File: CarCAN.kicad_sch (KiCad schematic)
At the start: 17 parts, among them J2 CAN_OUT, U4 ADM3055E, U5 CDSOT23-T24CAN

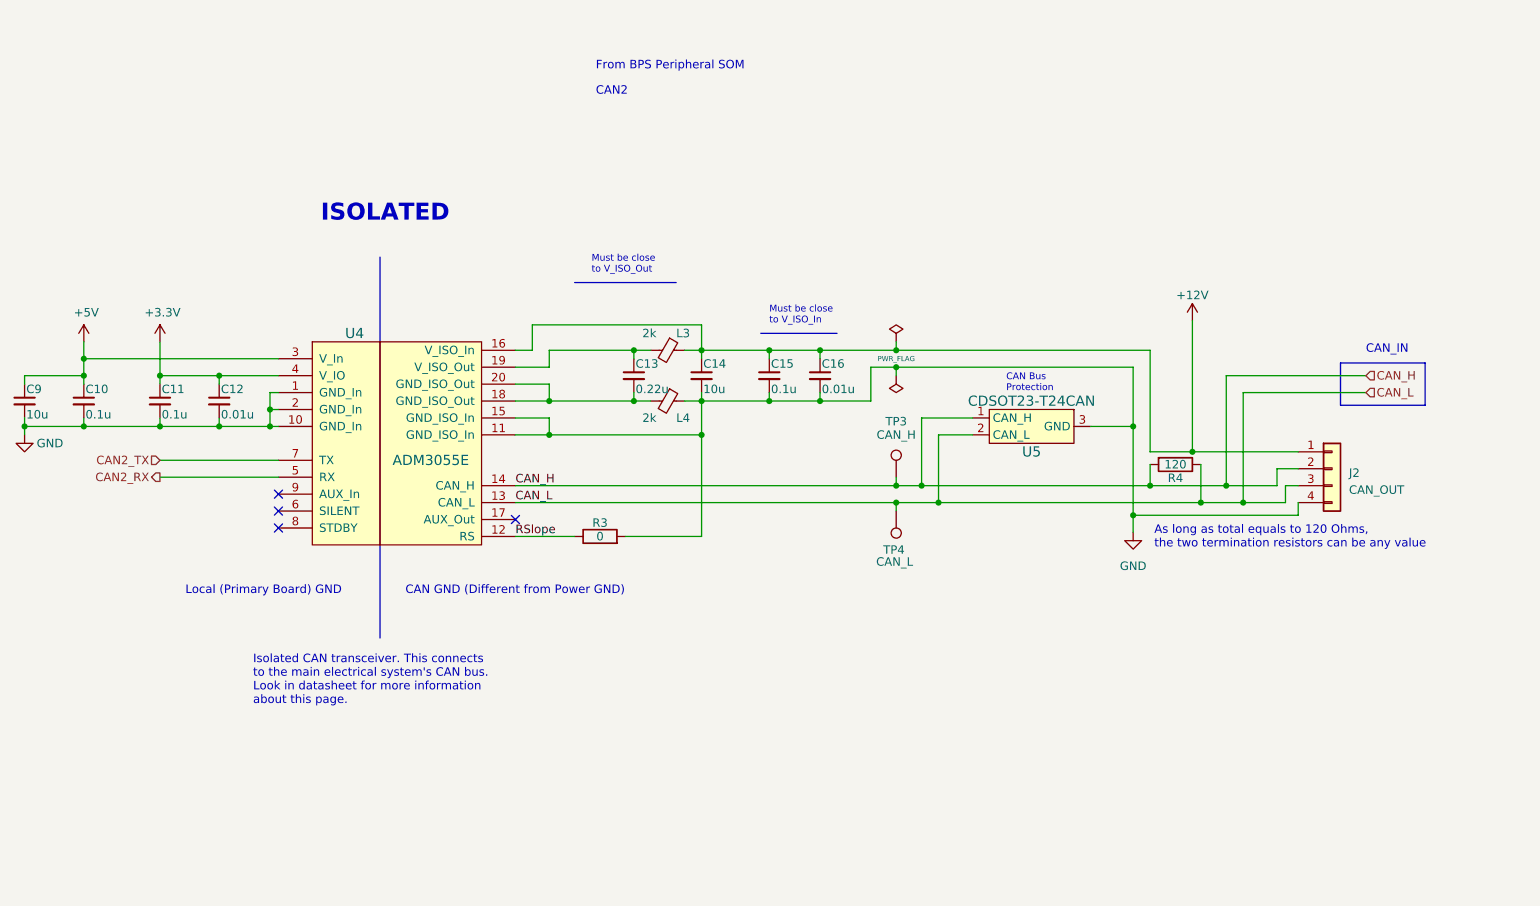
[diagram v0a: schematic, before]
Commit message: Updated pinouts and added protection circuitry for signals
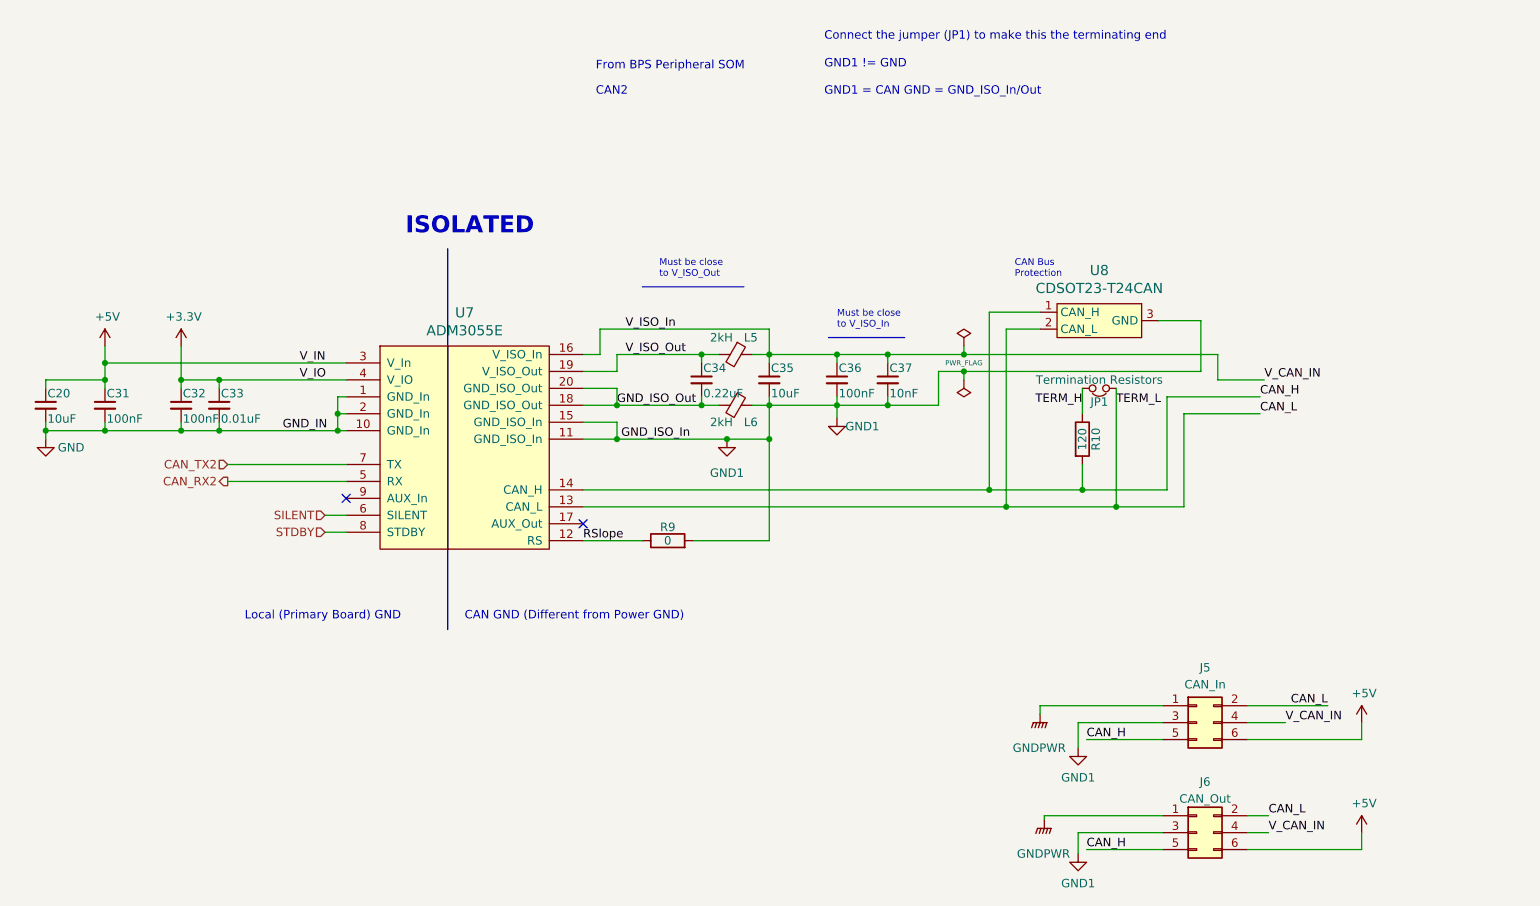
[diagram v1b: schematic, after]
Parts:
- removed C10, C11, C15: 0.1u, Capacitor_SMD:C_0805_2012Metric, symbol Device:C_Small
- removed C12, C16: 0.01u, Capacitor_SMD:C_0805_2012Metric, symbol Device:C_Small
- removed C13: 0.22u, Capacitor_SMD:C_0805_2012Metric, symbol Device:C_Small
- removed C14, C9: 10u, Capacitor_SMD:C_0805_2012Metric, symbol Device:C_Small
- removed J2: CAN_OUT, UTSVT_Connectors:Molex_MicroFit3.0_1x4xP3.00mm_PolarizingPeg_Vertical, symbol Connector_Generic:Conn_01x04
- removed L3, L4: 2k, Inductor_SMD:L_0805_2012Metric, symbol Device:FerriteBead_Small
- removed R3: 0, Resistor_SMD:R_0805_2012Metric, symbol Device:R
- removed R4: 120, Resistor_SMD:R_0805_2012Metric, symbol Device:R
- removed TP3: CAN_H, TestPoint:TestPoint_Keystone_5005-5009_Compact, symbol Connector:TestPoint
- removed TP4: CAN_L, TestPoint:TestPoint_Keystone_5005-5009_Compact, symbol Connector:TestPoint
- removed U4: ADM3055E, UTSVT_ICs:SOIC-20W_7.5x15.4mm_Pitch1.27mm, symbol utsvt-chips:ADM3055E
- removed U5: CDSOT23-T24CAN, Package_TO_SOT_SMD:SOT-23W, symbol utsvt-chips:CDSOT23-T24CAN
- added C20, C35: 10uF, Capacitor_SMD:C_0805_2012Metric, symbol Device:C_Small
- added C31, C32, C36: 100nF, Capacitor_SMD:C_0805_2012Metric, symbol Device:C_Small
- added C33: 0.01uF, Capacitor_SMD:C_0805_2012Metric, symbol Device:C_Small
- added C34: 0.22uF, Capacitor_SMD:C_0805_2012Metric, symbol Device:C_Small
- added C37: 10nF, Capacitor_SMD:C_0805_2012Metric, symbol Device:C_Small
- added J5: CAN_In, Connector_Molex:Molex_Micro-Fit_3.0_43045-0612_2x03_P3.00mm_Vertical, symbol Connector_Generic:Conn_02x03_Odd_Even
- added J6: CAN_Out, Connector_Molex:Molex_Micro-Fit_3.0_43045-0612_2x03_P3.00mm_Vertical, symbol Connector_Generic:Conn_02x03_Odd_Even
- added JP1: Termination Resistors, Connector_PinHeader_2.54mm:PinHeader_1x02_P2.54mm_Vertical, symbol Device:Jumper_NC_Small
- added L5, L6: 2kH, Inductor_SMD:L_0805_2012Metric, symbol Device:Ferrite_Bead_Small
- added R10: 120, Resistor_SMD:R_0805_2012Metric, symbol Device:R
- added R9: 0, Resistor_SMD:R_0805_2012Metric, symbol Device:R
- added U7: ADM3055E, UTSVT_ICs:SOIC-20W_7.5x15.4mm_Pitch1.27mm, symbol Dashboard-rescue:ADM3055E-utsvt-chips
- added U8: CDSOT23-T24CAN, Package_TO_SOT_SMD:SOT-23W, symbol Dashboard-rescue:CDSOT23-T24CAN-utsvt-chips
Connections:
- net +3.3V: now also C32.1, C33.1, U7.4 (V_IO)
- net +5V: now also C20.1, C31.1, J5.6 (Pin_6), J6.6 (Pin_6), U7.3 (V_In)
- net CAN_H: now also J5.5 (Pin_5), J6.5 (Pin_5), R10.2, U7.14 (CAN_H), U8.1 (CAN_H)
- net CAN_L: now also J5.2 (Pin_2), J6.2 (Pin_2), JP1.1, U7.13 (CAN_L), U8.2 (CAN_L)
- net GND: now also C20.2, C31.2, C32.2, C33.2, U7.1 (GND_In), U7.10 (GND_In), U7.2 (GND_In)
- net RSlope: now also R9.1, U7.12 (RS)
- new net CAN_RX2: U7.5 (RX)
- new net CAN_TX2: U7.7 (TX)
- new net GND1: C35.2, C36.2, C37.2, J5.3 (Pin_3), J6.3 (Pin_3), L6.1, R9.2, U7.11 (GND_ISO_In), U7.15 (GND_ISO_In), U8.3 (GND)
- new net GNDPWR: J5.1 (Pin_1), J6.1 (Pin_1)
- new net GND_ISO_Out: C34.2, L6.2, U7.18 (GND_ISO_Out), U7.20 (GND_ISO_Out)
- new net SILENT: U7.6 (SILENT)
- new net STDBY: U7.8 (STDBY)
- new net TERM_H: JP1.2, R10.1
- new net V_CAN_IN: C35.1, C36.1, C37.1, J5.4 (Pin_4), J6.4 (Pin_4), L5.1, U7.16 (V_ISO_In)
- new net V_ISO_Out: C34.1, L5.2, U7.19 (V_ISO_Out)
- no-connect marks 4 -> 2
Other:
- note added: "Connect the jumper (JP1) to make this the terminating end"
- note added: "GND1 != GND GND1 = CAN GND = GND_ISO_In/Out"
- note removed: "As long as total equals to 120 Ohms, the two termination resistors can be any value"
- note removed: "CAN_IN"
- note removed: "Isolated CAN transceiver. This connects to the main electrical system's CAN bus. Look in datasheet for more information about this page."

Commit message: Updated power distribution design
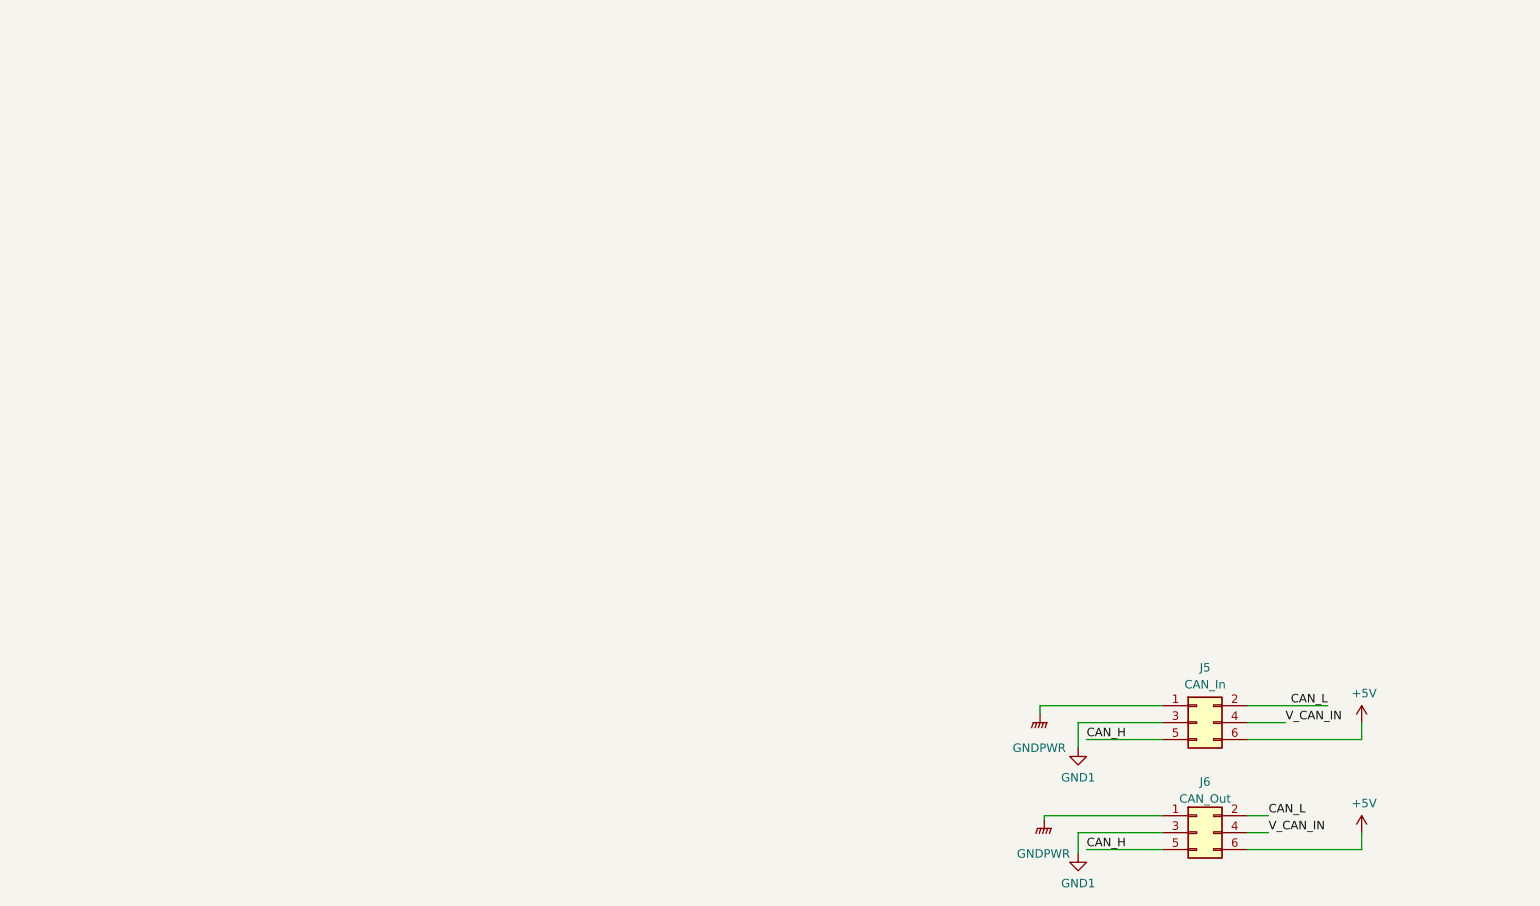
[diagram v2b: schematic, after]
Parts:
- removed C20, C35: 10uF, Capacitor_SMD:C_0805_2012Metric, symbol Device:C_Small
- removed C31, C32, C36: 100nF, Capacitor_SMD:C_0805_2012Metric, symbol Device:C_Small
- removed C33: 0.01uF, Capacitor_SMD:C_0805_2012Metric, symbol Device:C_Small
- removed C34: 0.22uF, Capacitor_SMD:C_0805_2012Metric, symbol Device:C_Small
- removed C37: 10nF, Capacitor_SMD:C_0805_2012Metric, symbol Device:C_Small
- removed JP1: Termination Resistors, Connector_PinHeader_2.54mm:PinHeader_1x02_P2.54mm_Vertical, symbol Device:Jumper_NC_Small
- removed L5, L6: 2kH, Inductor_SMD:L_0805_2012Metric, symbol Device:Ferrite_Bead_Small
- removed R10: 120, Resistor_SMD:R_0805_2012Metric, symbol Device:R
- removed R9: 0, Resistor_SMD:R_0805_2012Metric, symbol Device:R
- removed U7: ADM3055E, UTSVT_ICs:SOIC-20W_7.5x15.4mm_Pitch1.27mm, symbol Dashboard-rescue:ADM3055E-utsvt-chips
- removed U8: CDSOT23-T24CAN, Package_TO_SOT_SMD:SOT-23W, symbol Dashboard-rescue:CDSOT23-T24CAN-utsvt-chips
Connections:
- no-connect marks 2 -> 0
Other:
- note removed: "CAN Bus Protection"
- note removed: "CAN GND (Different from Power GND)"
- note removed: "CAN2"
- note removed: "Connect the jumper (JP1) to make this the terminating end"
- note removed: "From BPS Peripheral SOM"
- note removed: "GND1 != GND GND1 = CAN GND = GND_ISO_In/Out"
- note removed: "ISOLATED"
- note removed: "Local (Primary Board) GND"
- note removed: "Must be close to V_ISO_In"
- note removed: "Must be close to V_ISO_Out"

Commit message: Updated CAN circuitry and used new power protection PMOS
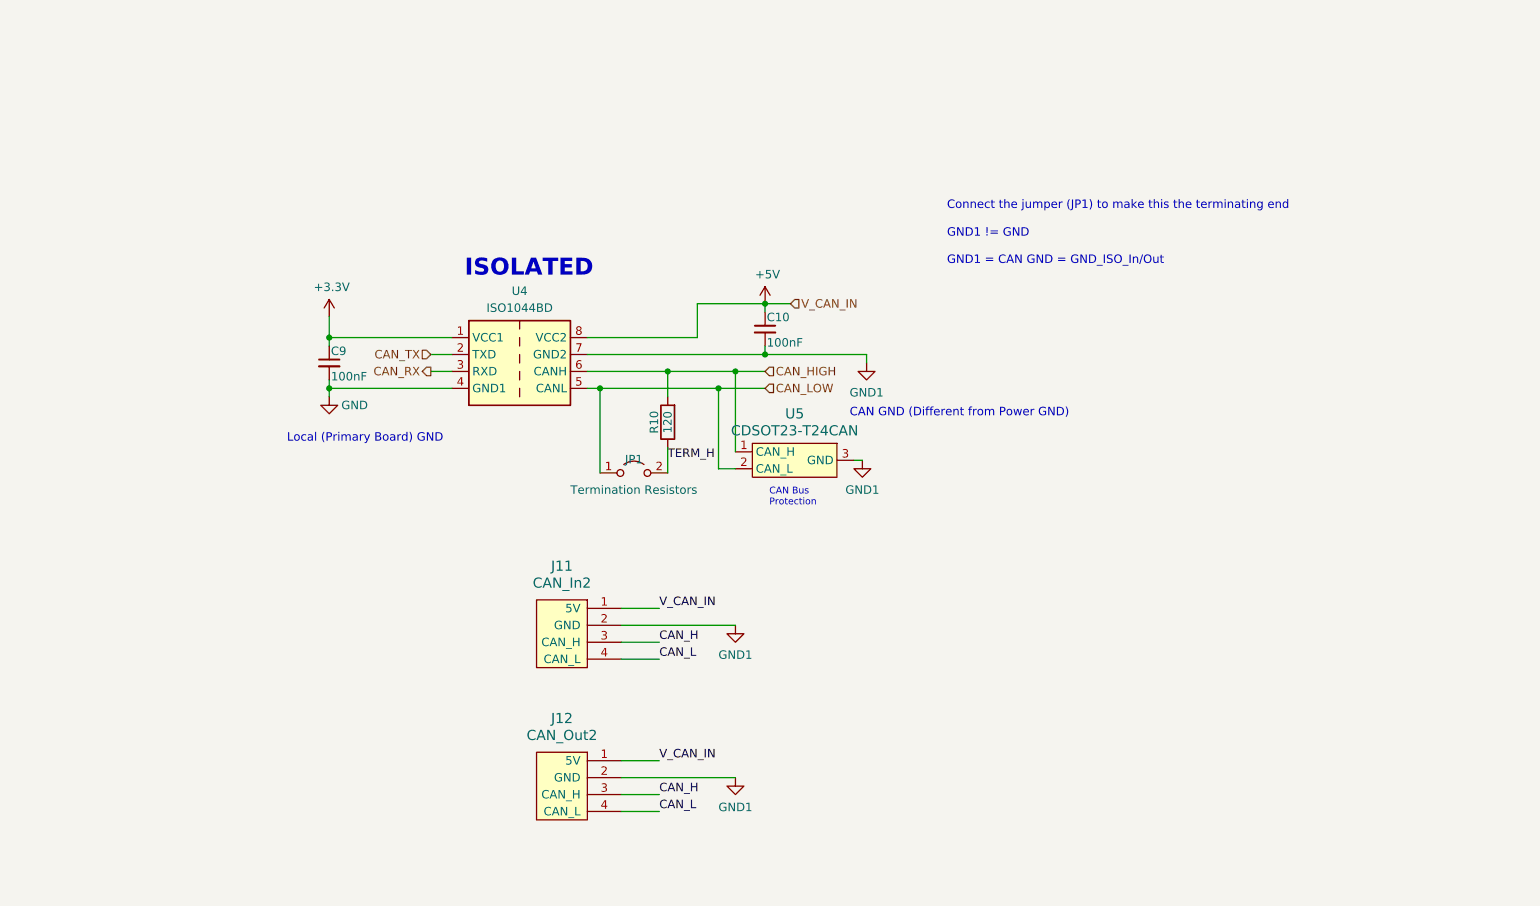
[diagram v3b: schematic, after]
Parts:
- removed J5: CAN_In, Connector_Molex:Molex_Micro-Fit_3.0_43045-0612_2x03_P3.00mm_Vertical, symbol Connector_Generic:Conn_02x03_Odd_Even
- removed J6: CAN_Out, Connector_Molex:Molex_Micro-Fit_3.0_43045-0612_2x03_P3.00mm_Vertical, symbol Connector_Generic:Conn_02x03_Odd_Even
- added C10, C9: 100nF, Capacitor_SMD:C_0805_2012Metric, symbol Device:C_Small
- added J11: CAN_In2, symbol utsvt-connectors:CANConnector
- added J12: CAN_Out2, symbol utsvt-connectors:CANConnector
- added JP1: Termination Resistors, Connector_PinHeader_2.54mm:PinHeader_1x02_P2.54mm_Vertical, symbol Jumper:Jumper_2_Open
- added R10: 120, Resistor_SMD:R_0805_2012Metric, symbol Device:R
- added U4: ISO1044BD, Package_SO:SSOP-8_3.9x5.05mm_P1.27mm, symbol utsvt-chips:ISO1044BD
- added U5: CDSOT23-T24CAN, Package_TO_SOT_SMD:SOT-23W, symbol utsvt-chips:CDSOT23-T24CAN
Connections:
- net +5V: now also C10.1, J11.1 (5V), J12.1 (5V), U4.8 (VCC2)
- net CAN_H: now also J11.3 (CAN_H), J12.3 (CAN_H)
- net CAN_L: now also J11.4 (CAN_L), J12.4 (CAN_L)
- net GND1: now also C10.2, J11.2 (GND), J12.2 (GND), U4.7 (GND2), U5.3 (GND)
- new net +3.3V: C9.1, U4.1 (VCC1)
- new net CAN_HIGH: R10.2, U4.6 (CANH), U5.1 (CAN_H)
- new net CAN_LOW: JP1.1 (A), U4.5 (CANL), U5.2 (CAN_L)
- new net CAN_RX: U4.3 (RXD)
- new net CAN_TX: U4.2 (TXD)
- new net GND: C9.2, U4.4 (GND1)
- new net TERM_H: JP1.2 (B), R10.1
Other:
- note added: "CAN Bus Protection"
- note added: "CAN GND (Different from Power GND)"
- note added: "Connect the jumper (JP1) to make this the terminating end"
- note added: "GND1 != GND GND1 = CAN GND = GND_ISO_In/Out"
- note added: "ISOLATED"
- note added: "Local (Primary Board) GND"

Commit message: Finished CAN circuitry
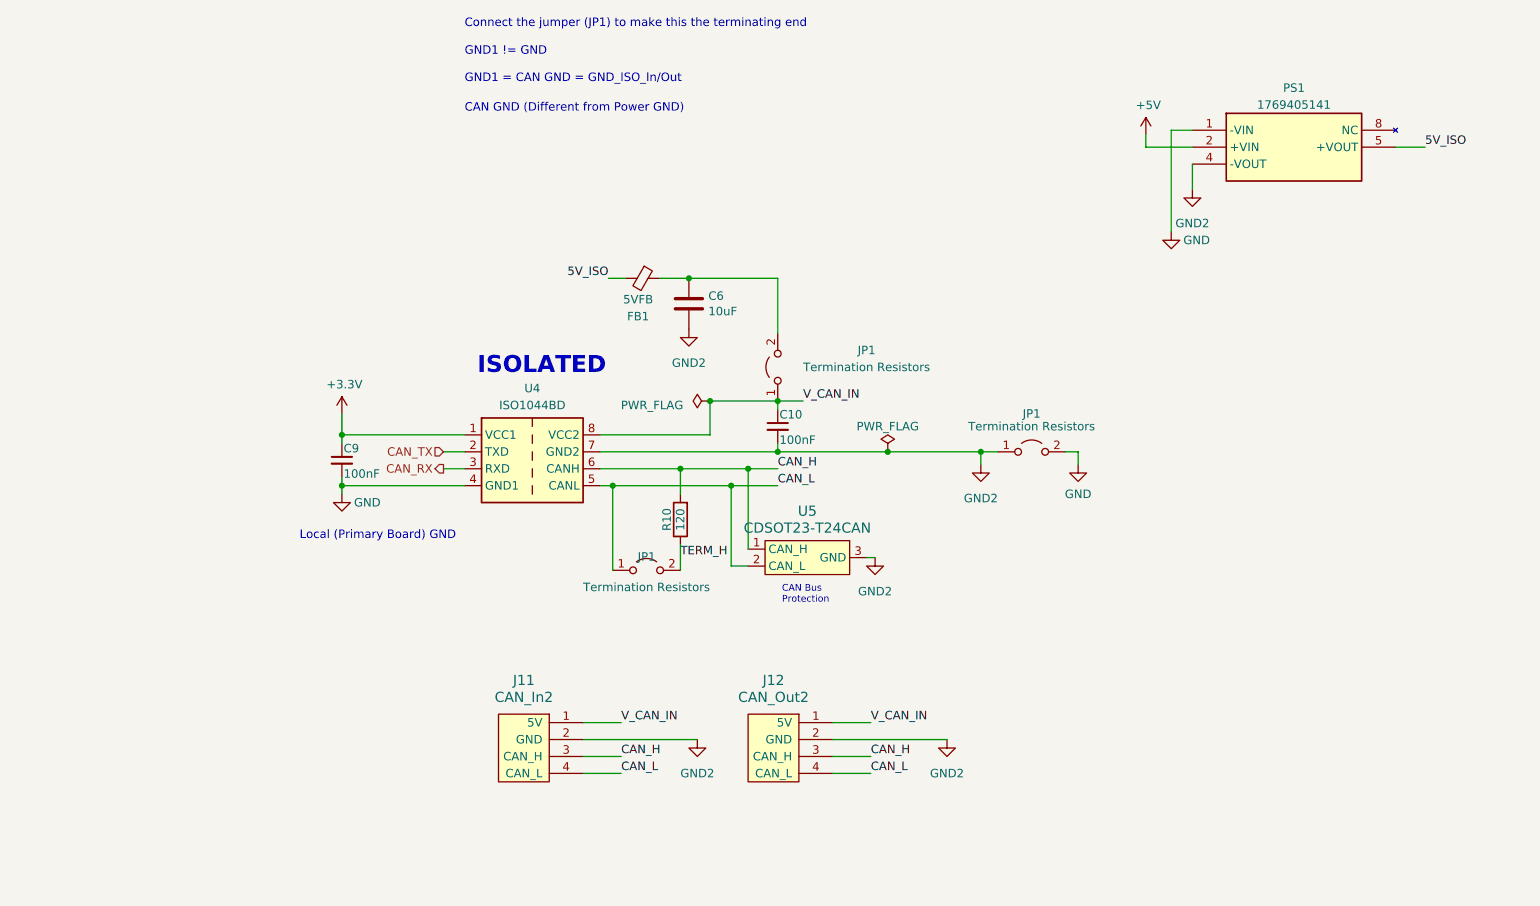
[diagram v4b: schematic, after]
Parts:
- added C6: 10uF, Capacitor_SMD:C_0805_2012Metric, symbol Device:C
- added FB1: 5VFB, Inductor_SMD:L_0805_2012Metric, symbol Device:FerriteBead_Small
- added JP1 (x2): Termination Resistors, Connector_PinHeader_2.54mm:PinHeader_1x02_P2.54mm_Vertical, symbol Jumper:Jumper_2_Open
- added PS1: 1769405141, 1769405141, symbol UTSVT_LeaderSOM:1769405141
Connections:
- net CAN_HIGH is gone; now on net CAN_H: R10.2, U4.6 (CANH), U5.1 (CAN_H)
- net CAN_LOW is gone; now on net CAN_L: JP1.1 (A), U4.5 (CANL), U5.2 (CAN_L)
- net +5V: now also PS1.2 (+VIN); no longer C10.1, J11.1 (5V), J12.1 (5V), U4.8 (VCC2)
- net GND: now also JP1.2 (B), PS1.1 (-VIN)
- net GND1 renamed GND2
- net GND2: now also C6.2, JP1.1 (A), PS1.4 (-VOUT)
- new net: C6.1, FB1.1, JP1.2 (B)
- new net 5V_ISO: FB1.2, PS1.5 (+VOUT)
- new net V_CAN_IN: C10.1, J11.1 (5V), J12.1 (5V), JP1.1 (A), U4.8 (VCC2)
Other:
- moved on the sheet: C10, C9, J11, J12, JP1, R10, U4, U5
